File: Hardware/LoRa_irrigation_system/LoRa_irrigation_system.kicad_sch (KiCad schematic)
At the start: 1 part, among them J1 12VIN

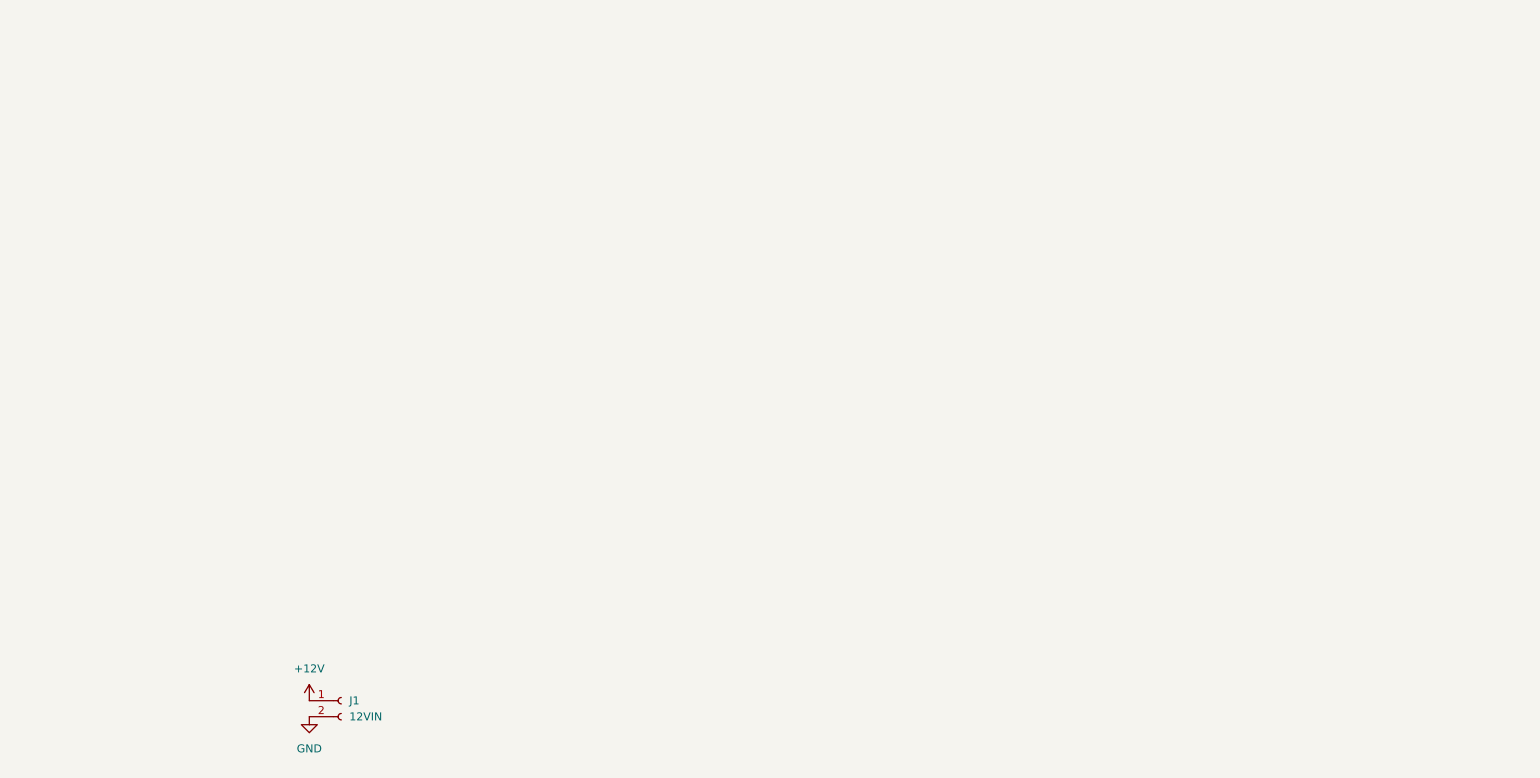
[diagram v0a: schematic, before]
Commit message: Sschematic design
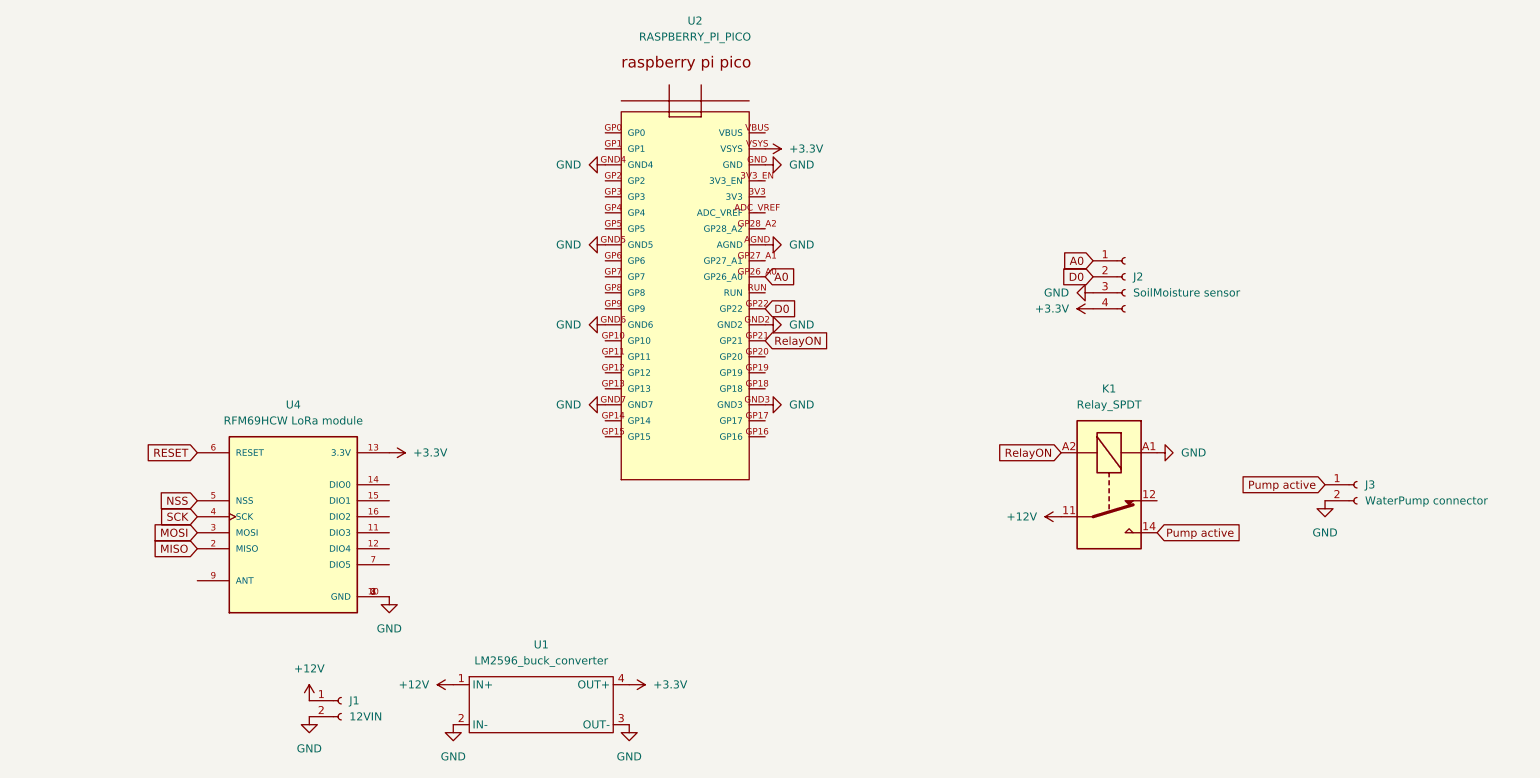
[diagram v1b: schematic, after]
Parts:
- added J2: SoilMoisture sensor, symbol Connector:Conn_01x04_Socket
- added J3: WaterPump connector, symbol Connector:Conn_01x02_Socket
- added K1: Relay_SPDT, symbol Relay:Relay_SPDT
- added U1: LM2596_buck_converter, symbol My_Symbols:LM2596_buck_converter
- added U2: RASPBERRY_PI_PICO, RASPBERRY_PI_PICO:RASPBERRY_PI_PICO, symbol RASPBERRY_PI_PICO:RASPBERRY_PI_PICO
- added U4: RFM69HCW LoRa module, COM-13909:MOD_COM-13909, symbol COM-13909:RFM69HCW LoRa module
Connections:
- net +12V: now also K1.11, U1.1 (IN+)
- net GND: now also J2.3 (Pin_3), J3.2 (Pin_2), K1.A1, U1.2 (IN-), U1.3 (OUT-), U2.AGND, U2.GND, U2.GND2, U2.GND3, U2.GND4, U2.GND5, U2.GND6, U2.GND7, U4.1 (GND), U4.10 (GND), U4.8 (GND)
- new net +3.3V: J2.4 (Pin_4), U1.4 (OUT+), U2.VSYS, U4.13 (3.3V)
- new net A0: J2.1 (Pin_1), U2.GP26_A0
- new net D0: J2.2 (Pin_2), U2.GP22
- new net MISO: U4.2 (MISO)
- new net MOSI: U4.3 (MOSI)
- new net NSS: U4.5 (NSS)
- new net Pump active: J3.1 (Pin_1), K1.14
- new net RESET: U4.6 (RESET)
- new net RelayON: K1.A2, U2.GP21
- new net SCK: U4.4 (SCK)

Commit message: SCH complete*
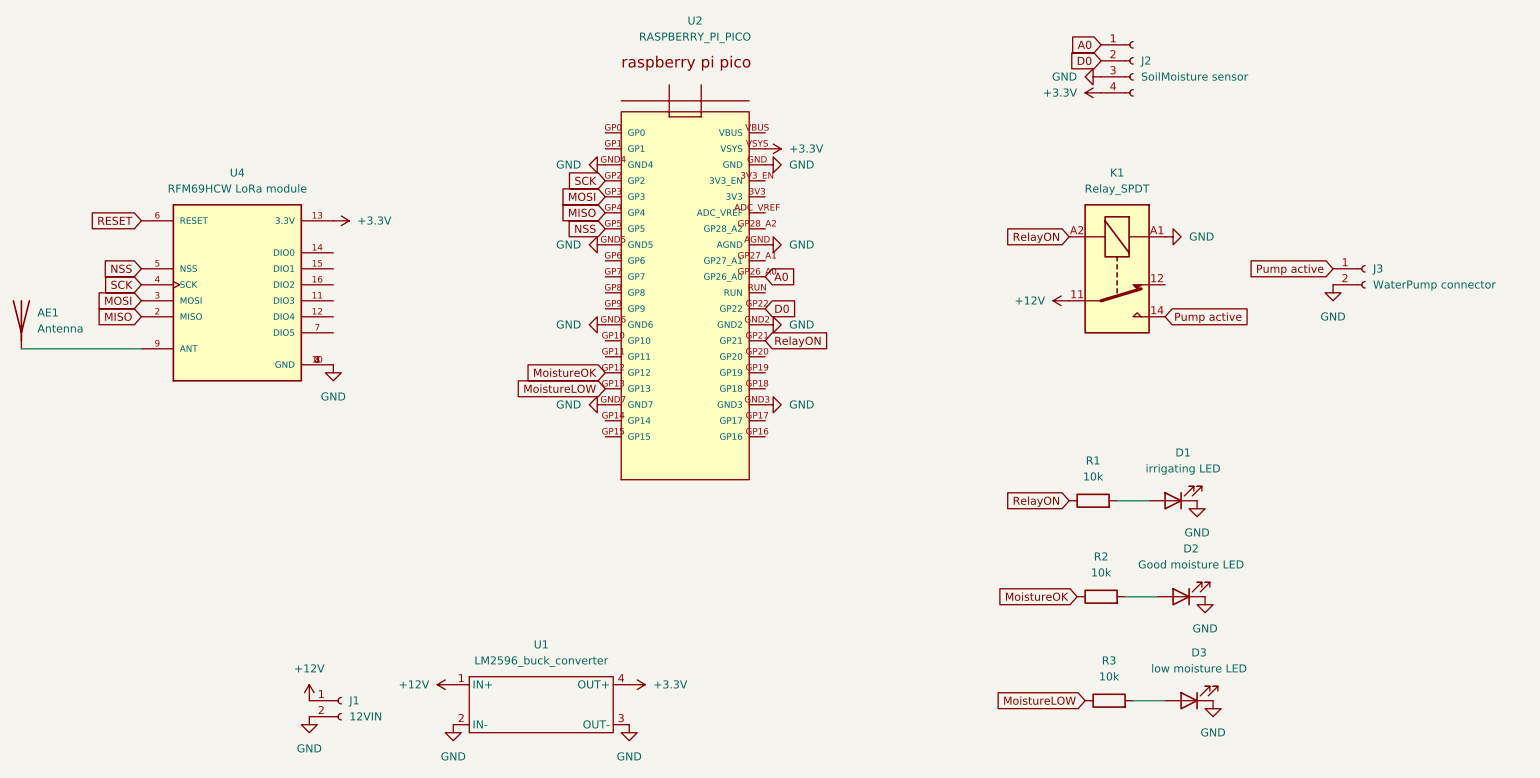
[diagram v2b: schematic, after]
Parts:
- added AE1: Antenna, symbol Device:Antenna
- added D1: irrigating LED, symbol Device:LED
- added D2: Good moisture LED, symbol Device:LED
- added D3: low moisture LED, symbol Device:LED
- added R1, R2, R3: 10k, symbol Device:R
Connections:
- net GND: now also D1.1 (K), D2.1 (K), D3.1 (K)
- net MISO: now also U2.GP4
- net MOSI: now also U2.GP3
- net NSS: now also U2.GP5
- net RelayON: now also R1.1
- net SCK: now also U2.GP2
- net at U4.9 (ANT): now also AE1.1 (A)
- net MoistureOK: now reaches U2.GP12
- net MoistureOK: now also R2.1
- net MoistureLOW: now reaches U2.GP13
- net MoistureLOW: now also R3.1
- new net: D1.2 (A), R1.2
- new net: D2.2 (A), R2.2
- new net: D3.2 (A), R3.2
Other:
- moved on the sheet: J2, J3, K1, U4
